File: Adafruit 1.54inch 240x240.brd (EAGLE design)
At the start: 40.6 x 41.9 mm, 23 parts, among them IC1 4050D, IC2 AP2112, Q2 MICROSD, Q3 BSS138

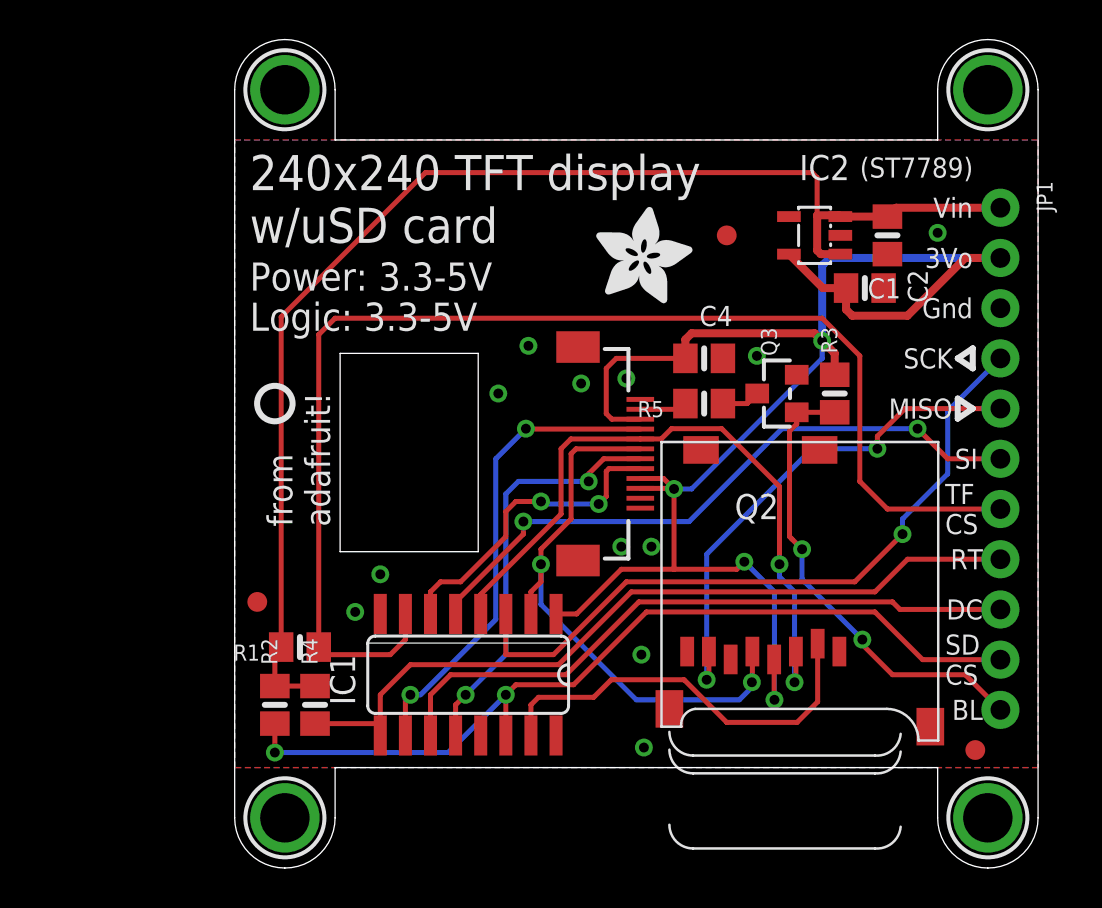
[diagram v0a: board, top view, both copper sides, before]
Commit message: Updating board files.
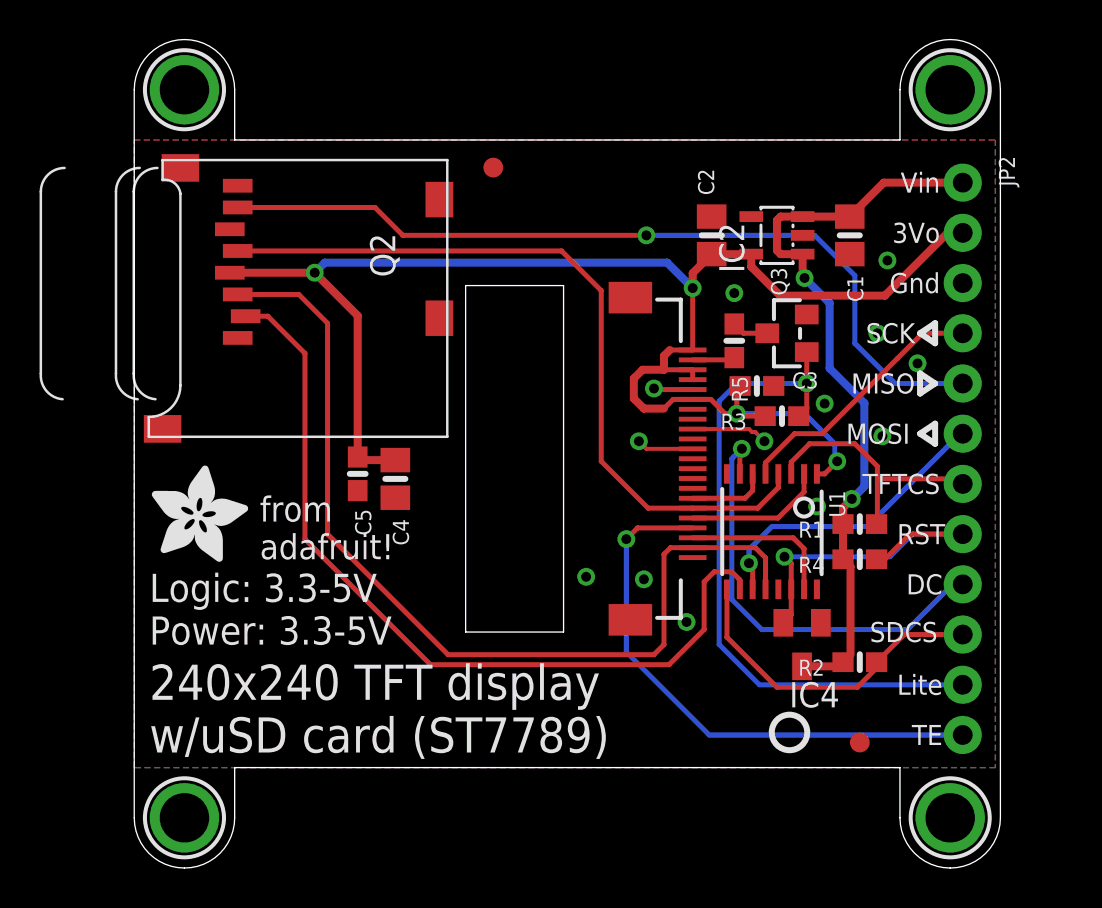
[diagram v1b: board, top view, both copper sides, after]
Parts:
- removed DISP1: DISP_LCD_ST7789_1.54IN, microbuilder:TFT_1.54IN_240X240
- removed IC1: 4050D, 40xx:SO16
- removed JP1: (no value), microbuilder:1X11_ROUND_76
- removed U$3: FIDUCIAL_1MM, microbuilder:FIDUCIAL_1MM
- added C3, C5: 0.1uF, microbuilder:0603-NO
- added IC4: APX803-SAG, adafruit:SOT23
- added JP2: (no value), microbuilder:1X12_ROUND_76MIL
- added TFT1: DISP_TFT_1.54IN_240X240_22P, microbuilder:TFT_1.54IN_240X240_22PIN
- added U1: 74HC4050PWR, microbuilder:TSSOP16
- C4: value 0.1uF -> 10uF
- R1, R2, R4, R5: device microbuilder:0805-NO -> microbuilder:0603-NO
- R3: value 2.2K -> 10K; device microbuilder:0805-NO -> microbuilder:0603-NO
- moved U$2 30.9 mm to (28.1, 1.78), turned to 180 degrees
- moved R2 29.7 mm to (31.6, 5.33), turned to 180 degrees
- moved R1 29.0 mm to (31.6, 12.3)
- moved R4 28.5 mm to (31.6, 10.5), turned to 180 degrees
- moved U$5 26.5 mm to (31.6, 1.27)
- moved U$1 26.0 mm to (-4.19, 10.4)
- moved U$4 25.0 mm to (13.1, 30.4)
- moved Q2 17.9 mm to (10.8, 30.7), turned to 270 degrees
- moved C4 16.8 mm to (8.13, 14.6), turned to 270 degrees
- moved C2 8.19 mm to (24.1, 26.9), turned to 90 degrees
- moved U$7 5.08 mm to (-2.54, 34.3)
- moved U$8 5.08 mm to (-2.54, -2.54)
- moved R5 3.52 mm to (25.3, 21.6), turned to 270 degrees
- moved Q3 3.09 mm to (27.9, 22.0)
- moved R3 2.90 mm to (27.7, 17.8), turned to 180 degrees
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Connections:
- new net TE: JP2.12, TFT1.19
- net +3V3: now also C3.1, C5.1, JP2.2, TFT1.1, TFT1.3, TFT1.4, TFT1.6, U1.1; no longer DISP1.10, DISP1.3, DISP1.9, IC1.1, JP1.2
- net CARDCS: now also JP2.10, U1.9; no longer IC1.14, JP1.10
- net CARDCS_3V: now also U1.10; no longer IC1.15
- net GND: now also C3.2, C5.2, IC4.1, JP2.3, TFT1.10, TFT1.11, TFT1.12, TFT1.13, TFT1.14, TFT1.15, TFT1.22, TFT1.5, TFT1.7, TFT1.8, TFT1.9, TFT1.SUPPORT1, TFT1.SUPPORT2, U1.8; no longer DISP1.1, DISP1.11, DISP1.12, DISP1.SUPPORT1, DISP1.SUPPORT2, IC1.8, JP1.3
- net LEDK: now also TFT1.2; no longer DISP1.2
- net LITE: now also JP2.11; no longer JP1.11
- net MISO: now also JP2.5; no longer JP1.5
- net MOSI: now also JP2.6, U1.11; no longer IC1.5, JP1.6
- net MOSI_3V: now also TFT1.21, U1.12; no longer DISP1.5, IC1.4
- net SCK: now also JP2.4, U1.5; no longer IC1.3, JP1.4
- net SCK_3V: now also TFT1.17, U1.4; no longer DISP1.6, IC1.2
- net TFTCS: now also JP2.7, U1.3; no longer IC1.7, JP1.7
- net TFTCS_3V: now also TFT1.18, U1.2; no longer DISP1.8, IC1.6
- net TFTDC: now also JP2.9, U1.7; no longer IC1.11, JP1.9
- net TFTDC_3V: now also TFT1.16, U1.6; no longer DISP1.7, IC1.12
- net TFTRST: now also IC4.2, JP2.8, U1.14; no longer IC1.9, JP1.8
- net TFTRST_3V: now also TFT1.20, U1.15; no longer DISP1.4, IC1.10
- net VIN: now also IC4.3, JP2.1; no longer JP1.1
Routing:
- net TFTCS: track 64.5 -> 13.2 mm
- net TE: track 0.00 -> 28.1 mm, vias 0 -> 1
- net CARDCS: track 44.2 -> 16.7 mm, vias 2 -> 0
- net VIN: track 65.5 -> 38.6 mm, vias 0 -> 2
- net SCK: track 35.6 -> 13.3 mm, vias 1 -> 0
- net TFTRST: track 40.2 -> 18.0 mm, vias 0 -> 1
- net CARDCS_3V: track 20.8 -> 41.8 mm
- net MOSI: track 32.8 -> 15.3 mm, vias 2 -> 1
- net TFTDC_3V: track 21.3 -> 4.04 mm, vias 2 -> 0
- net MISO: track 26.1 -> 42.4 mm, vias 2 -> 1
- net TFTRST_3V: track 24.1 -> 7.92 mm, vias 2 -> 0
- net MOSI_3V: track 34.5 -> 47.2 mm, vias 2 -> 0
- net TFTDC: track 33.0 -> 22.4 mm, vias 0 -> 1
- net LITE: track 23.7 -> 33.7 mm, vias 2 -> 1
- net SCK_3V: track 29.3 -> 38.9 mm, vias 2 -> 0
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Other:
- board size 40.6 x 41.9 mm -> 43.8 x 41.9 mm
- board text added: "1.54" ST7789 240x240"
- board text added: "CK"
- board text added: "Lite"
- board text added: "MOSI"
- board text added: "RST"
- board text added: "SDCS"
- board text added: "TE"
- board text added: "TFTCS"
- board text added: "V+"
- board text added: "w/uSD card (ST7789)"
- board text removed: "(ST7789)"
- board text removed: "CL"
- board text removed: "SD CS"
- board text removed: "TF CS"
- board text removed: "Vi"
- board text removed: "w/uSD card"
